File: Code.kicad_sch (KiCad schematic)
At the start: 8 parts

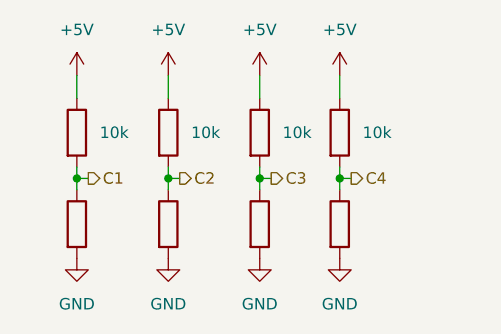
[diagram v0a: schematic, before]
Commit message: Started PCB Work
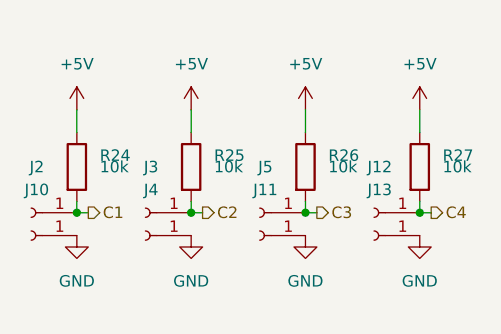
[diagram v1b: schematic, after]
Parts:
- removed R22, R24, R28: ~, symbol Device:R
- removed R23: 10k, symbol Device:R
- added J10, J11, J12, J13, J2, J3, J4, J5: Conn_01x01_Socket, Connector_PinSocket_1.27mm:PinSocket_1x01_P1.27mm_Vertical, symbol Connector:Conn_01x01_Socket
- R24: renamed from R21; footprint (none) -> Resistor_SMD:R_0805_2012Metric_Pad1.20x1.40mm_HandSolder
- R25, R27: footprint (none) -> Resistor_SMD:R_0805_2012Metric_Pad1.20x1.40mm_HandSolder
- R26: value ~ -> 10k; footprint (none) -> Resistor_SMD:R_0805_2012Metric_Pad1.20x1.40mm_HandSolder
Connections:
- net +5V: now also R26.1
- net C1: now also J2.1 (Pin_1)
- net C2: now also R25.2, J3.1 (Pin_1)
- net C3: now also R26.2, J5.1 (Pin_1); no longer R25.2, R26.1
- net C4: now also J12.1 (Pin_1)
- net GND: now also J10.1 (Pin_1), J11.1 (Pin_1), J13.1 (Pin_1), J4.1 (Pin_1); no longer R26.2
